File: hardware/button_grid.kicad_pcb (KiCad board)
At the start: 2 copper layers, 393.9 x 175.4 mm, 434 parts, among them J2 TFT 2.4in, J3 USB-C, J4 USB D+/D-, U1 MCP23S17, U2 MCP23S17, U3 MPR121, U3 Teensy 4.1, U4 MPR121

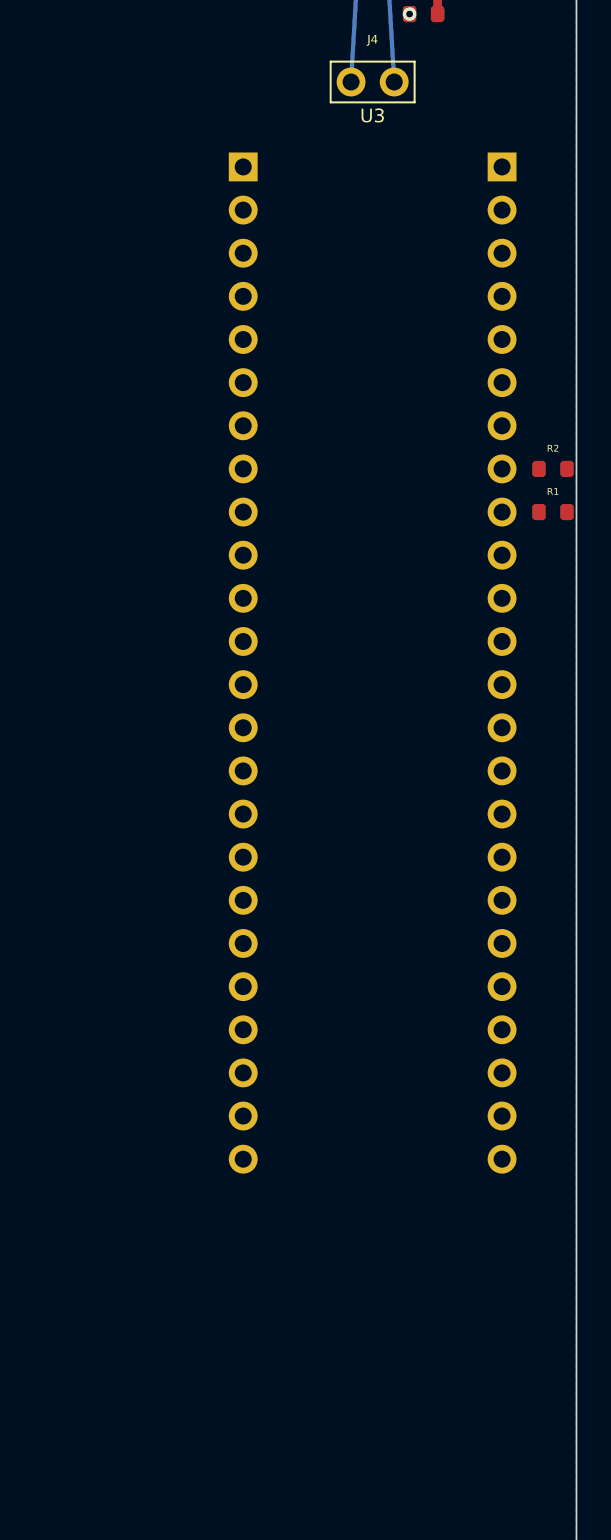
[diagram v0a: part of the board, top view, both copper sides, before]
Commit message: Generate latest version kicad file
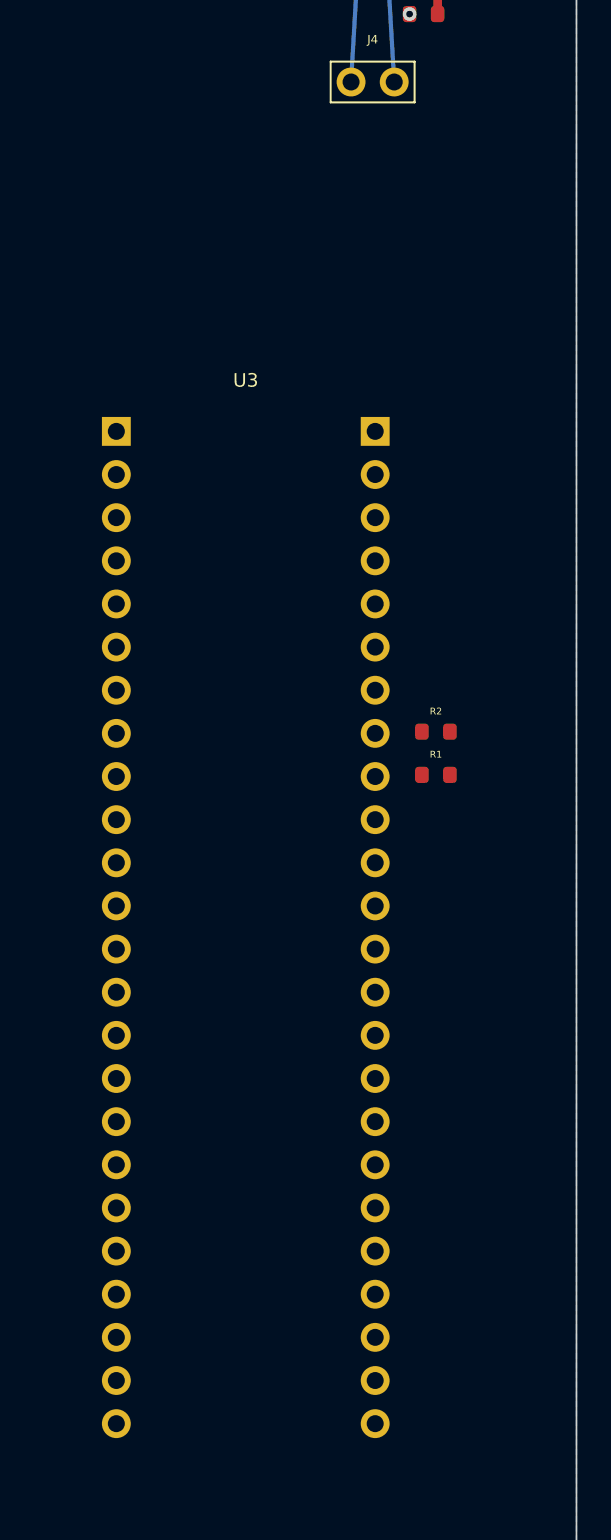
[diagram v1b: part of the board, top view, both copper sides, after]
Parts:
- moved U3 17.3 mm to (374.4, 39.6)
- moved R1 16.9 mm to (385.6, 59.8)
- moved R2 16.9 mm to (385.6, 57.2)
